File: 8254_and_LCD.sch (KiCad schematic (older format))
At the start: 7 parts, among them J501 Conn_01x03_Male, J502 Conn_01x02_Male, J503 Conn_01x03_Male, U501 PAL16L8, U502 8254, U503 PAL16L8

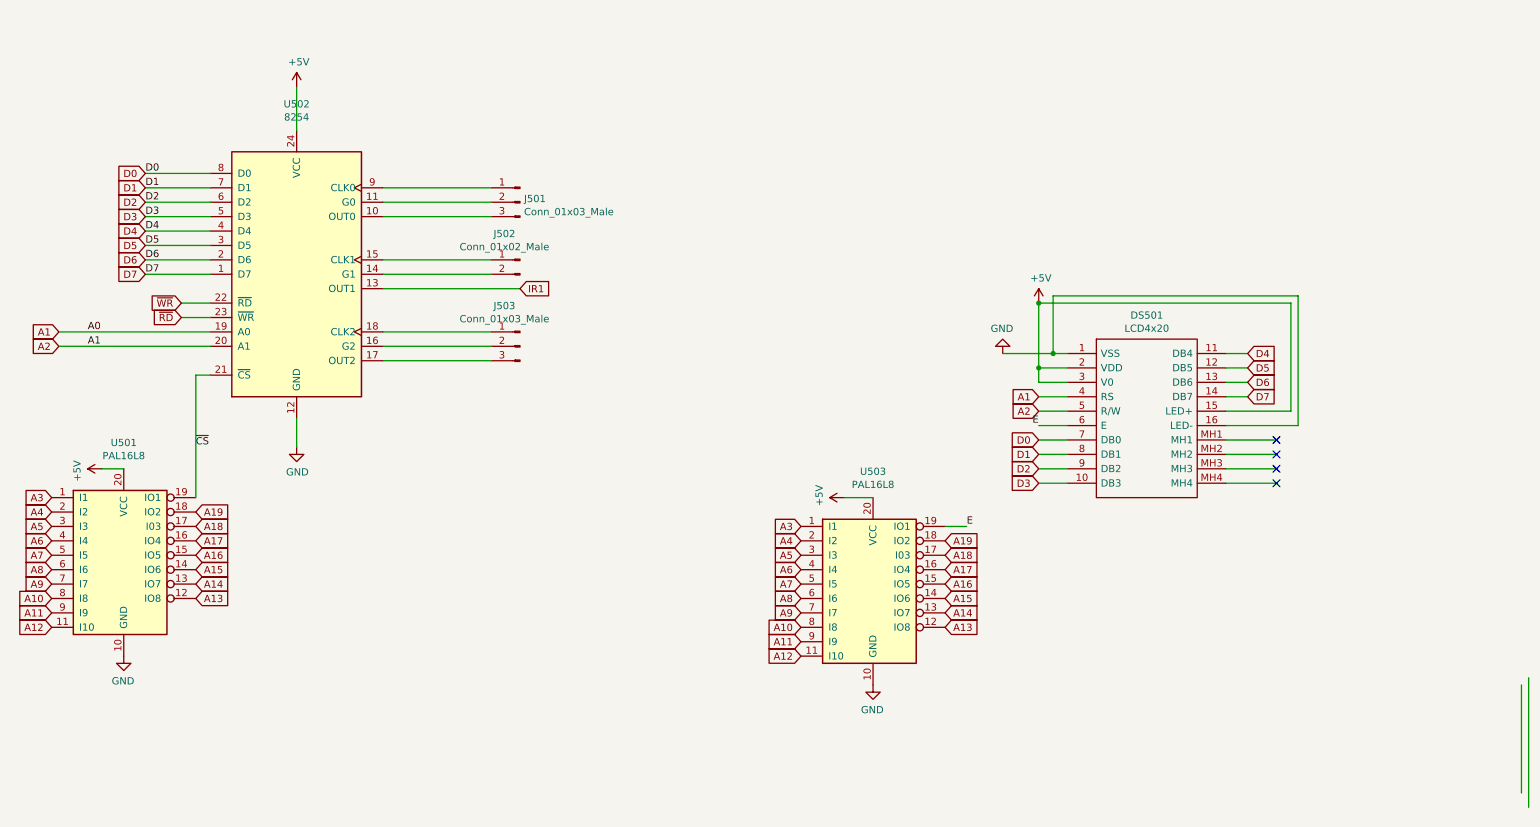
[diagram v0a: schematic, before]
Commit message: made some modifications
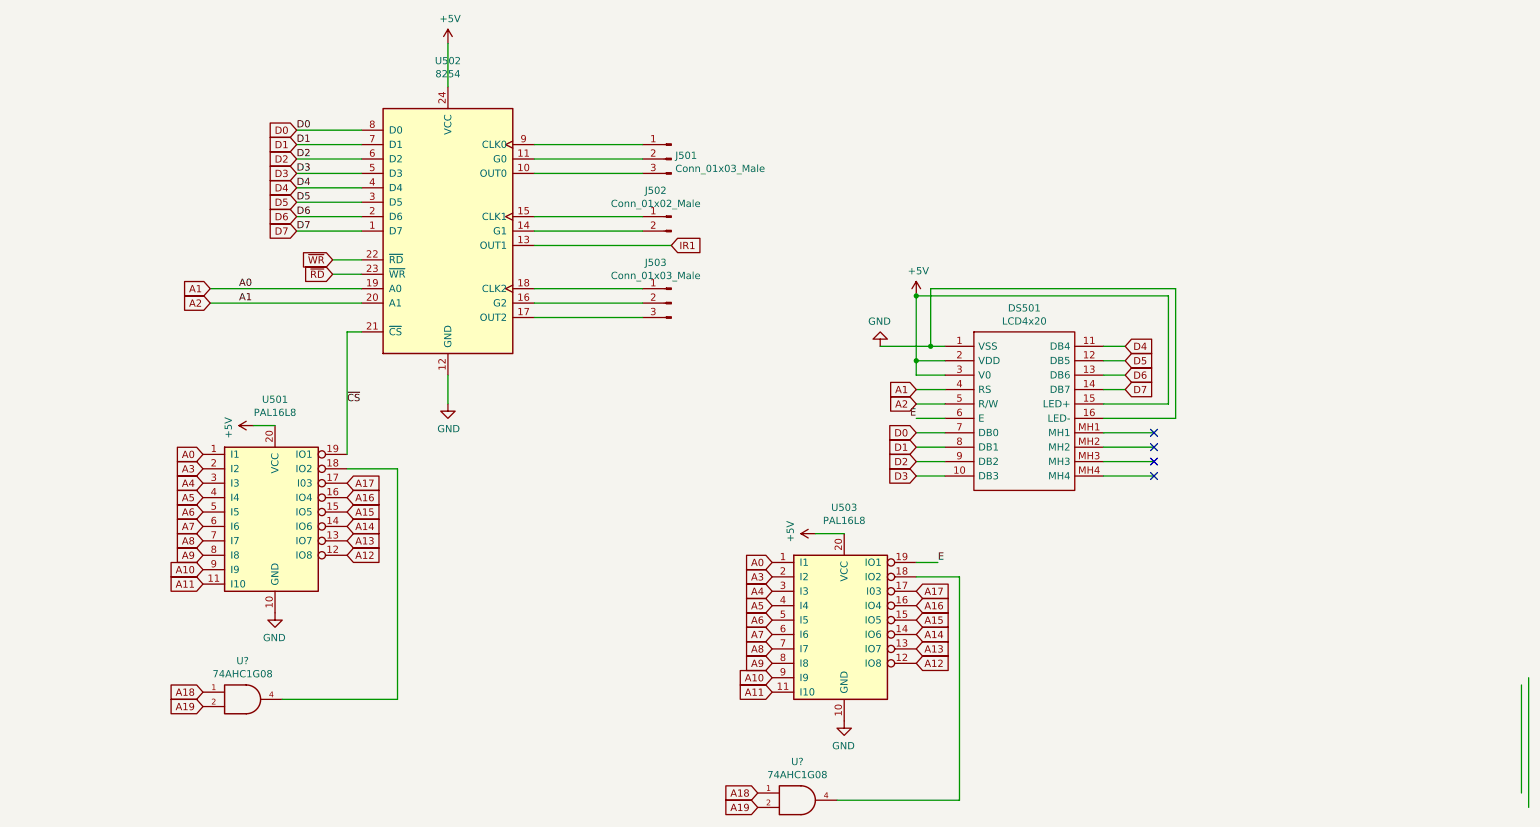
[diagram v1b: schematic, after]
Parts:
- added U? (x2): 74AHC1G08, symbol 74xGxx:74AHC1G08
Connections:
- wire segments 58 -> 64
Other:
- moved on the sheet: DS501, J501, J502, J503, U501, U502, U503
